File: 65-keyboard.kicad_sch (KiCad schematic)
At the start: 20 parts, among them SW1 SW_Push, U1 ATmega32U4-A, Y1 Crystal_GND24_Small

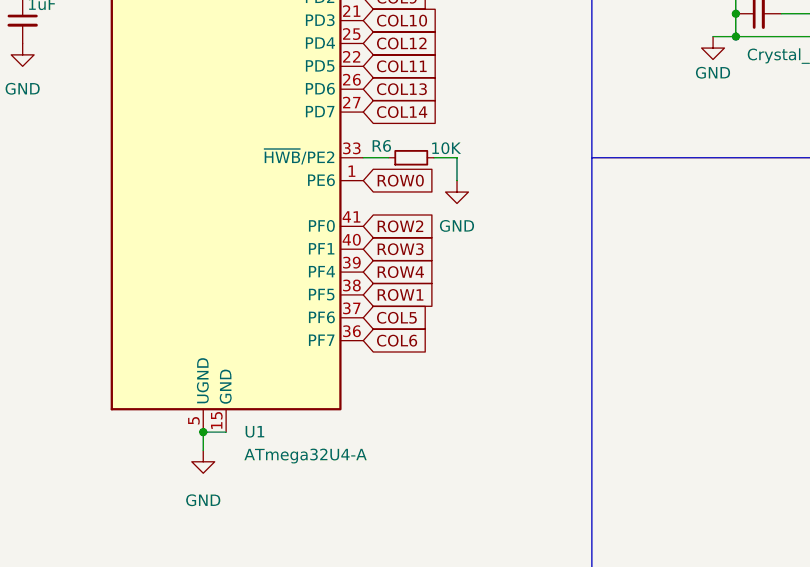
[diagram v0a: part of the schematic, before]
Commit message: more routing
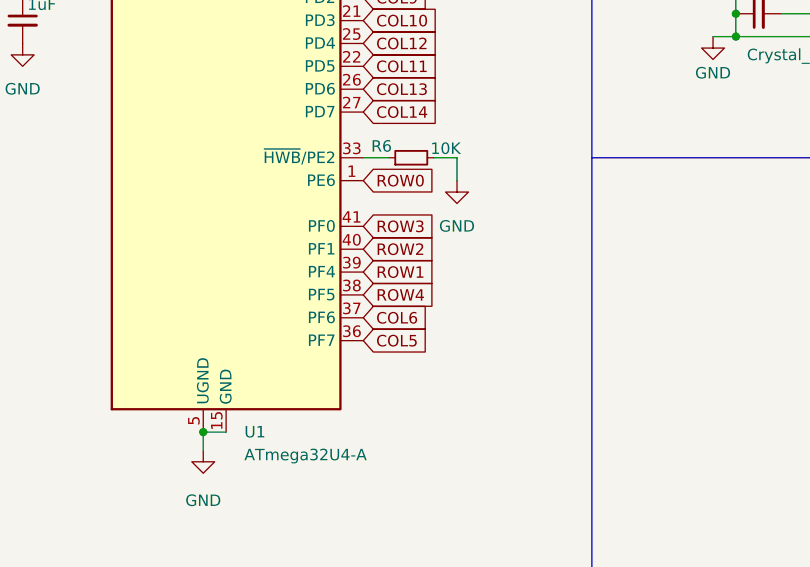
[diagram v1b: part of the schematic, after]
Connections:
- net COL5: now also U1.36 (PF7); no longer U1.37 (PF6)
- net COL6: now also U1.37 (PF6); no longer U1.36 (PF7)
- net ROW1: now also U1.39 (PF4); no longer U1.38 (PF5)
- net ROW2: now also U1.40 (PF1); no longer U1.41 (PF0)
- net ROW3: now also U1.41 (PF0); no longer U1.40 (PF1)
- net ROW4: now also U1.38 (PF5); no longer U1.39 (PF4)
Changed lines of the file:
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@@
     )
   )
-  (global_label "ROW4" (shape input) (at 70.358 96.52 0) (fields_autoplaced)
+  (global_label "ROW4" (shape input) (at 70.358 99.06 0) (fields_autoplaced)
     (effects (font (size 1.27 1.27)) (justify left))
-    (property "Intersheet References" "${INTERSHEET_REFS}" (id 0) (at 78.0325 96.4406 0)
+    (property "Intersheet References" "${INTERSHEET_REFS}" (id 0) (at 78.0325 98.9806 0)
       (effects (font (size 1.27 1.27)) (justify left) hide)
     )
   )
-  (global_label "COL5" (shape input) (at 70.358 101.6 0) (fields_autoplaced)
+  (global_label "COL5" (shape input) (at 70.358 104.14 0) (fields_autoplaced)
     (effects (font (size 1.27 1.27)) (justify left))
-    (property "Intersheet References" "${INTERSHEET_REFS}" (id 0) (at 77.6092 101.5206 0)
+    (property "Intersheet References" "${INTERSHEET_REFS}" (id 0) (at 77.6092 104.0606 0)
       (effects (font (size 1.27 1.27)) (justify left) hide)
     )
@@
     )
   )
-  (global_label "ROW3" (shape input) (at 70.358 93.98 0) (fields_autoplaced)
+  (global_label "ROW3" (shape input) (at 70.358 91.44 0) (fields_autoplaced)
     (effects (font (size 1.27 1.27)) (justify left))
-    (property "Intersheet References" "${INTERSHEET_REFS}" (id 0) (at 78.0325 93.9006 0)
+    (property "Intersheet References" "${INTERSHEET_REFS}" (id 0) (at 78.0325 91.3606 0)
       (effects (font (size 1.27 1.27)) (justify left) hide)
     )
@@
     )
   )
-  (global_label "COL6" (shape input) (at 70.358 104.14 0) (fields_autoplaced)
+  (global_label "COL6" (shape input) (at 70.358 101.6 0) (fields_autoplaced)
     (effects (font (size 1.27 1.27)) (justify left))
-    (property "Intersheet References" "${INTERSHEET_REFS}" (id 0) (at 77.6092 104.0606 0)
+    (property "Intersheet References" "${INTERSHEET_REFS}" (id 0) (at 77.6092 101.5206 0)
       (effects (font (size 1.27 1.27)) (justify left) hide)
     )
@@
     )
   )
-  (global_label "ROW1" (shape input) (at 70.358 99.06 0) (fields_autoplaced)
+  (global_label "ROW1" (shape input) (at 70.358 96.52 0) (fields_autoplaced)
     (effects (font (size 1.27 1.27)) (justify left))
-    (property "Intersheet References" "${INTERSHEET_REFS}" (id 0) (at 78.0325 98.9806 0)
+    (property "Intersheet References" "${INTERSHEET_REFS}" (id 0) (at 78.0325 96.4406 0)
       (effects (font (size 1.27 1.27)) (justify left) hide)
     )
@@
     )
   )
-  (global_label "ROW2" (shape input) (at 70.358 91.44 0) (fields_autoplaced)
+  (global_label "ROW2" (shape input) (at 70.358 93.98 0) (fields_autoplaced)
     (effects (font (size 1.27 1.27)) (justify left))
-    (property "Intersheet References" "${INTERSHEET_REFS}" (id 0) (at 78.0325 91.3606 0)
+    (property "Intersheet References" "${INTERSHEET_REFS}" (id 0) (at 78.0325 93.9006 0)
       (effects (font (size 1.27 1.27)) (justify left) hide)
     )
